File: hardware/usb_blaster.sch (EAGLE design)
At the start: 18 parts, among them IC2 PIC18F14K50SO, X1 53047-06

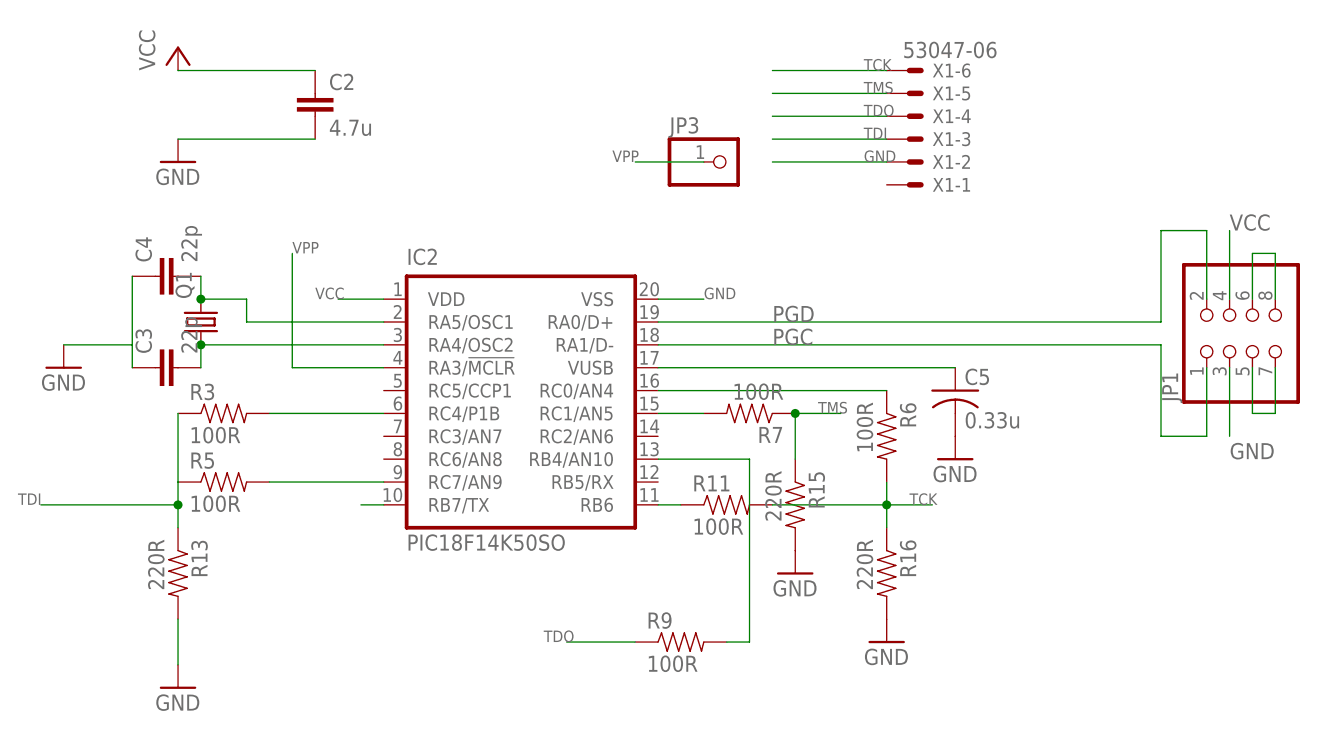
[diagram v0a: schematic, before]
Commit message: Añado splitter
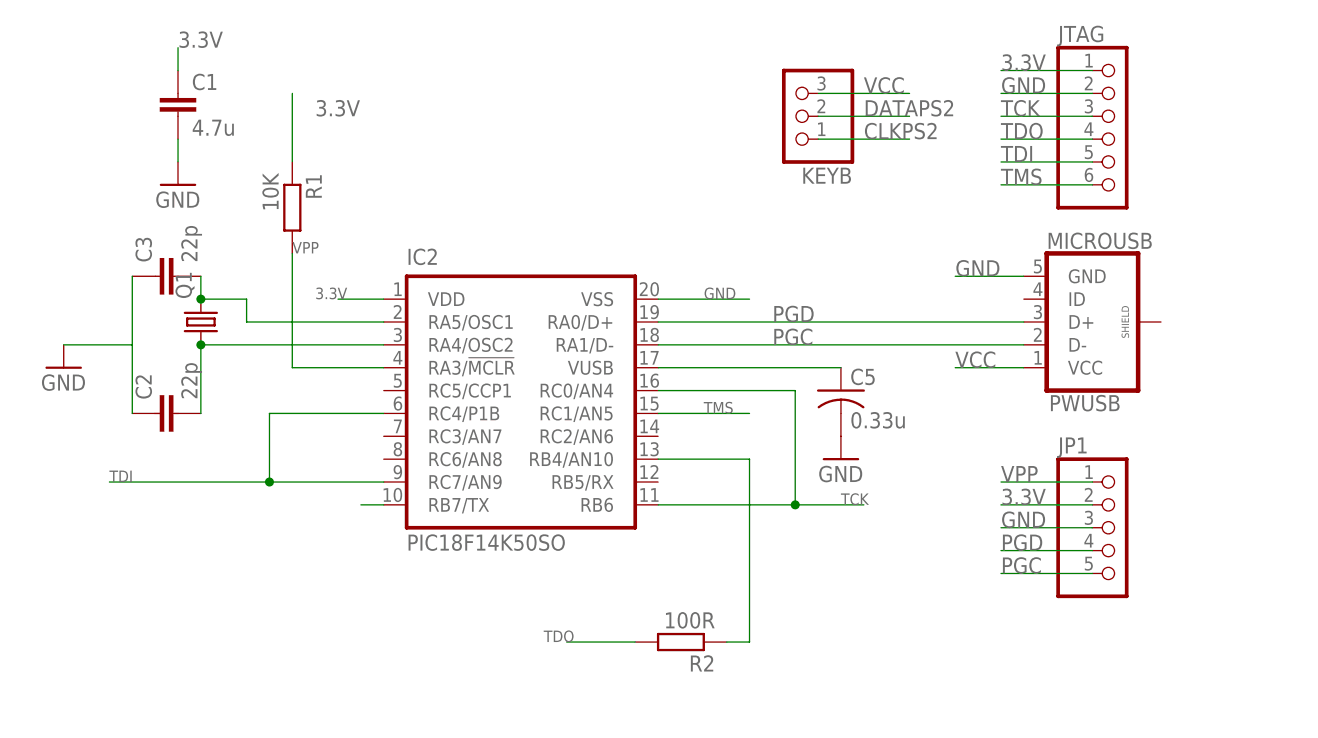
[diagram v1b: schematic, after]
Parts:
- removed C4: 22p, SparkFun:CAP0805
- removed JP3: (no value), pinhead:PINHD-1X1
- removed R11, R3, R5, R6, R7, R9: 100R, SparkFun:RESISTOR0805-RES
- removed R13, R15, R16: 220R, SparkFun:RESISTOR0805-RES
- removed X1: 53047-06, con-molex:53047-06
- added C1: 4.7u, rcl:C-EUC0805
- added JTAG: (no value), pinhead:PINHD-1X6
- added KEYB: (no value), pinhead:PINHD-1X3
- added PWUSB: MICROUSB, zxuno_rev_mcleod:MICROUSB
- added R1: 10K, rcl:R-EU_R0805
- added R2: 100R, rcl:R-EU_R0805
- C2: value 4.7u -> 22p; device SparkFun:CAP0805 -> rcl:C-EUC0805
- C3: device SparkFun:CAP0805 -> rcl:C-EUC0805
- C5: device rcl:C-USC0603K -> rcl:C-USC0805
- JP1: device pinhead:PINHD-2X4 -> pinhead:PINHD-1X5
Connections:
- removed net N$13: IC2.RC7/AN9, R5.2
- removed net N$16: IC2.RB6, R11.1
- removed net N$2: IC2.RC1/AN5, R7.2
- removed net N$3: JP1.6, JP1.8
- removed net N$5: JP1.5, JP1.7
- removed net N$6: IC2.RC0/AN4, R6.1
- removed net N$8: IC2.RC4/P1B, R3.2
- new net 3.3V: C1.1, IC2.VDD, JP1.2, JTAG.1, R1.1
- new net CLKPS2: KEYB.1
- new net DATAPS2: KEYB.2
- net GND: now also C1.2, C2.1, JTAG.2, PWUSB.GND; no longer C2.2, C4.1, R13.2, R15.2, R16.2, X1-2.S
- net N$1: now also C3.2; no longer C4.2
- net N$4: now also C2.2; no longer C3.2
- net N$7: now also R2.1; no longer R9.2
- net PGC: now also JP1.5, PWUSB.D-; no longer JP1.1
- net PGD: now also JP1.4, PWUSB.D+; no longer JP1.2
- net TCK: now also IC2.RB6, IC2.RC0/AN4, JTAG.3; no longer R11.2, R16.1, R6.2, X1-6.S
- net TDI: now also IC2.RC4/P1B, IC2.RC7/AN9, JTAG.5; no longer R13.1, R3.1, R5.1, X1-3.S
- net TDO: now also JTAG.4, R2.2; no longer R9.1, X1-4.S
- net TMS: now also IC2.RC1/AN5, JTAG.6; no longer R15.1, R7.1, X1-5.S
- net VCC: now also KEYB.3, PWUSB.VCC; no longer C2.1, IC2.VDD, JP1.4
- net VPP: now also JP1.1, R1.2; no longer JP3.1
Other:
- moved on the sheet: C2, C3, C5
